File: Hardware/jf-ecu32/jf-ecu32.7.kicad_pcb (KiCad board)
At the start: 2 copper layers, 71.3 x 48 mm, 106 parts, among them J1 GAZ, J10 k, J11 RPM, J12 S.PORT, J13 PPM/PWM, J14 PUMP1, J15 PUMP1, J16 PPM/PWM, J17 PUMP2, J18 PUMP2, J19 EN, J2 AUX, J22 Micro_SD_Card_Det1, J23 Conn_01x04, J24 Conn_01x05, J3 PPM/PWM, J4 STARTER, J5 GLOW, J6 VANNE KEROSTART, J7 VANNE KERO, J8 BATTERY 2S/3S, J9 STARTER, Q1 A49T, Q2 A49T, Q3 A49T, Q4 LR8726, Q5 LR8726, Q6 LR8726, Q7 A49T, Q8 A49T, Q9 FDD6685, U1 ESP32-WROOM-32D, U10 BMP280, U2 4050, U3 MAX31855KASA, U4 AMS1117-3.3, U5 4050, U6 AMS1117-5.0, U7 OPA340NA, U8 LM4040DBZ-2.5, U9 INA219AxDCN

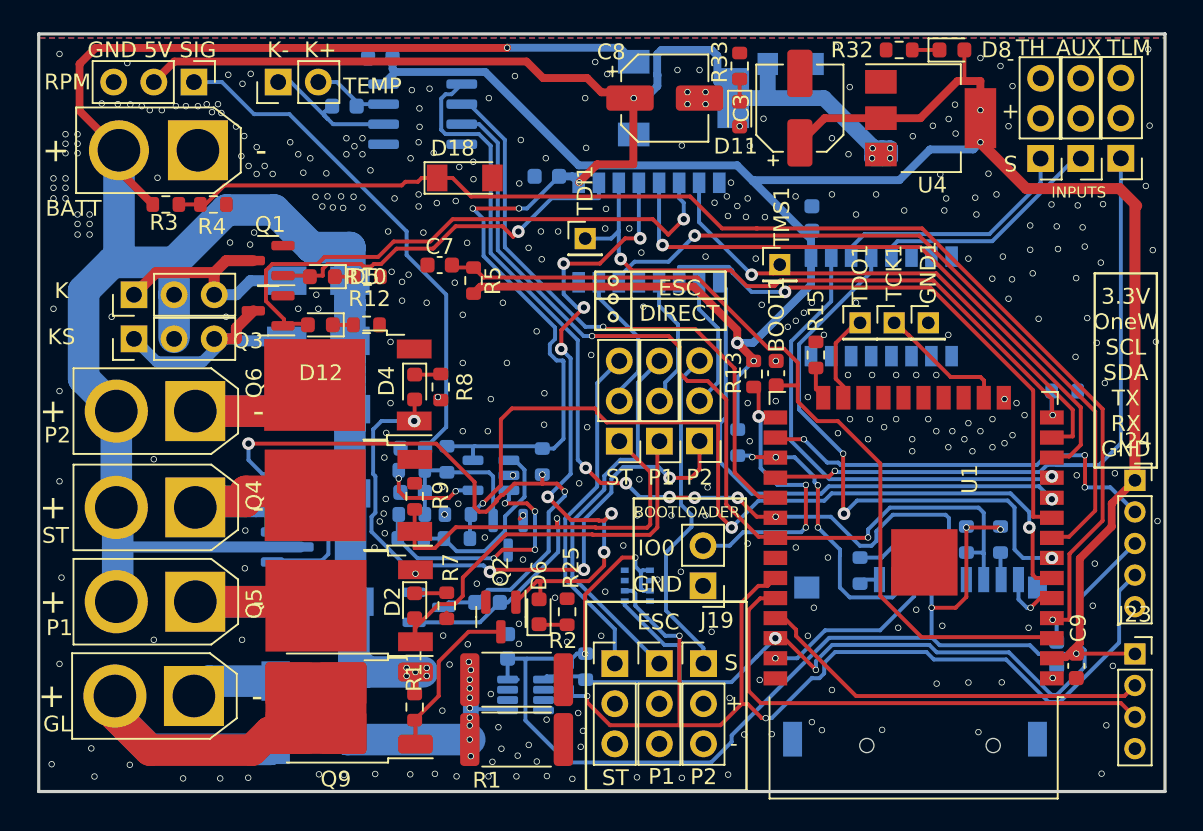
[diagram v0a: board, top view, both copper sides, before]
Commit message: PCB Update
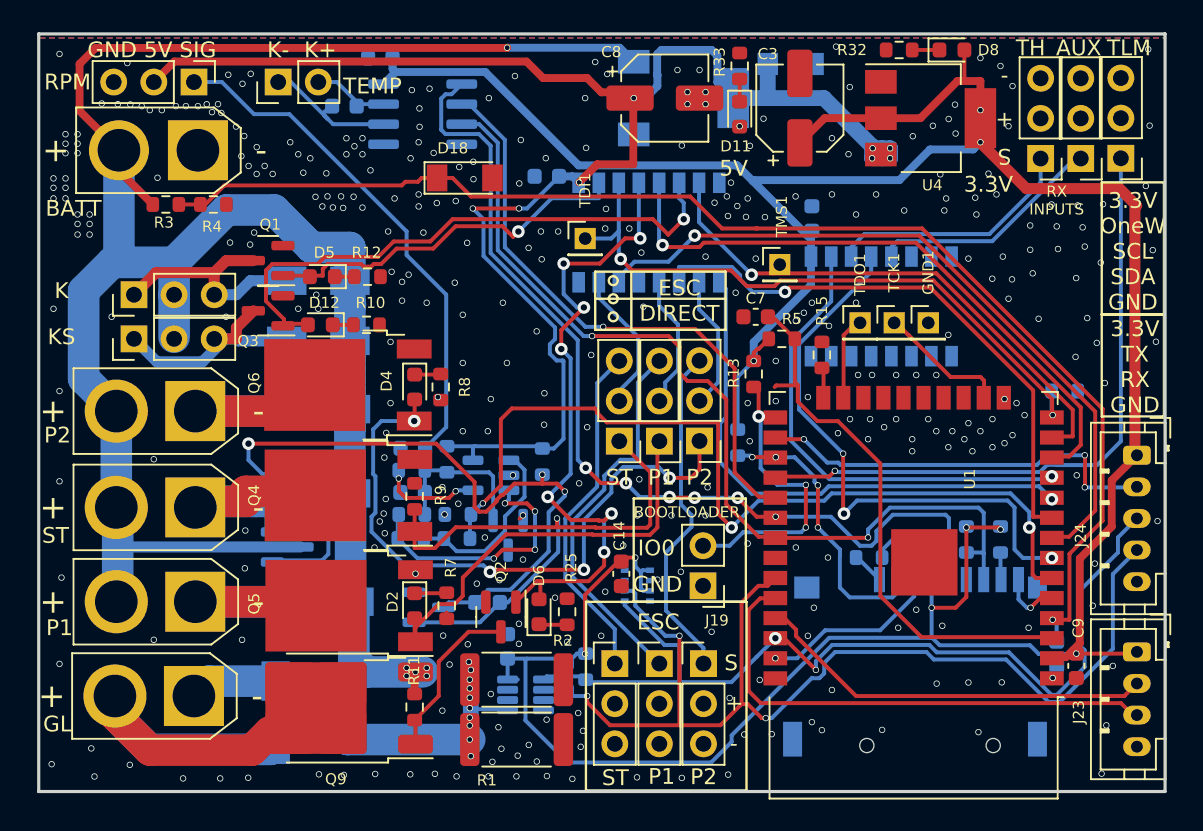
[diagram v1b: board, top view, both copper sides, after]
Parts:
- removed BOOT1: BOOT, Capacitor_SMD:C_0603_1608Metric
- added C14: 0.1µF, Capacitor_SMD:C_0603_1608Metric, F.Cu at (49.7, 184.3)
- J23: footprint Connector_PinSocket_2.00mm:PinSocket_1x04_P2.00mm_Vertical -> Connector_JST:JST_PH_B4B-PH-K_1x04_P2.00mm_Vertical
- J24: footprint Connector_PinSocket_2.00mm:PinSocket_1x05_P2.00mm_Vertical -> Connector_JST:JST_PH_B5B-PH-K_1x05_P2.00mm_Vertical
- moved C7 20.3 mm to (58.2, 168.0)
- moved R5 19.9 mm to (59.8, 169.4), turned to 0 degrees
- moved J24 1.59 mm to (82.3, 176.8), turned to -90 degrees
- moved R26 1.00 mm to (65.3, 183.3), turned to 0 degrees
- moved R15 0.38 mm to (62.4, 170.4)
- moved J23 0.18 mm to (82.3, 189.2), turned to -90 degrees
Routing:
- net Net-(U1-EN): track 55.6 -> 35.0 mm
- net 3.3V: track 234.3 -> 215.0 mm, vias 10 -> 9
- net ESP_SCL: track 55.9 -> 57.5 mm
- net ESP_SDA: track 68.2 -> 69.8 mm
- net Net-(J22-DAT2): track 1.33 -> 2.06 mm
- net OneWire: track 26.4 -> 25.9 mm
- net GND: vias 349 -> 347
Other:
- board text added: "3.3V"
- board text added: "3.3V OneW SCL SDA GND"
- board text added: "3.3V TX RX GND"
- board text added: "5V"
- board text added: "RX INPUTS"
- board text removed: "3.3V OneW SCL SDA TX RX GND"
- board text removed: "INPUTS"
- board text removed: "S + -"
